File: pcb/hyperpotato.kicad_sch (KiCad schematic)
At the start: 38 parts, among them J1 Conn_01x02_Socket, J2 Conn_01x03_Pin, Q1 AO3401A, SW1 SW_Push_45deg, SW10 SW_Push_45deg, SW11 SW_Push_45deg, SW12 SW_Push_45deg, SW13 SW_Push_45deg, SW14 SW_SPDT, SW15 SW_Push, SW2 SW_Push_45deg, SW3 SW_Push_45deg, SW4 SW_Push_45deg, SW5 SW_Push_45deg, SW6 SW_Push_45deg, SW7 SW_Push_45deg, SW8 SW_Push_45deg, SW9 SW_Push_45deg, U1 Seeeduino Xiao nRF52840, U2 SK8707-01-SENSOR, U3 SK8707-01, U4 DRV2605LDGS

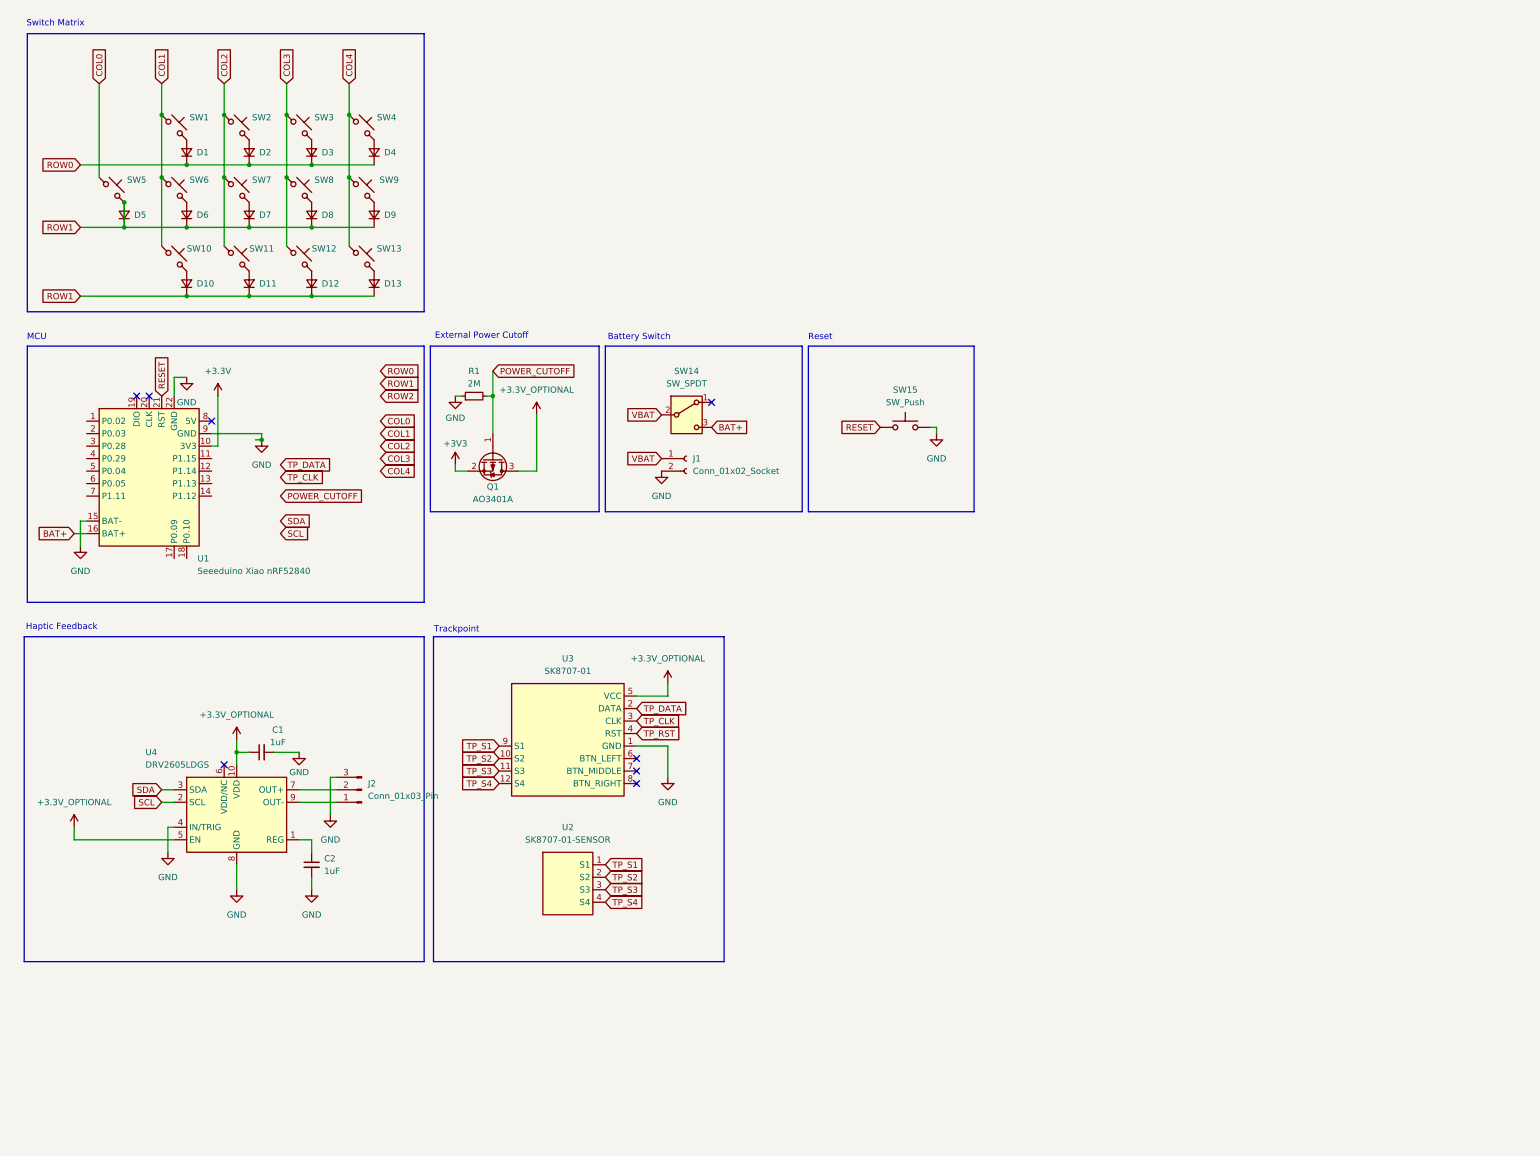
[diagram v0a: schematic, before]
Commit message: Start back with e73 module
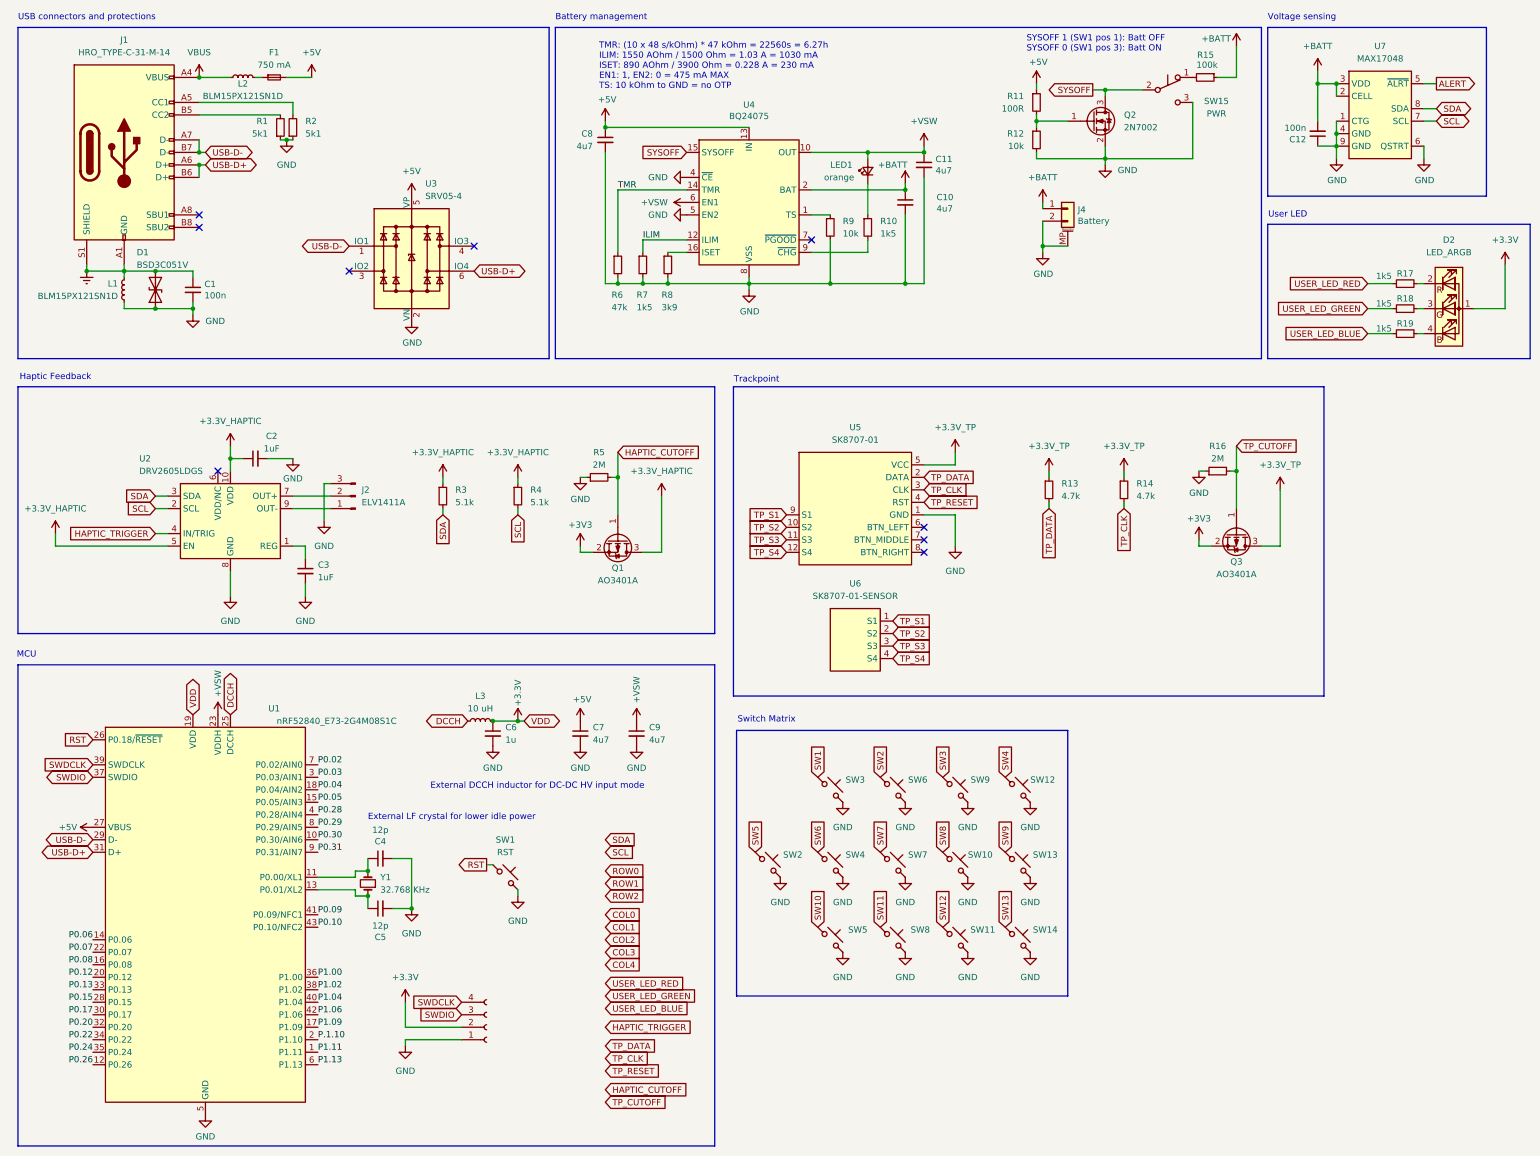
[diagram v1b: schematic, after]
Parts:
- removed D1, D10, D11, D12, D13, D2, D3, D4, D5, D6, D7, D8, D9: D_Small, ssbb_parts:D_1206_HandSolder_reversible, symbol Device:D_Small
- removed J1: Conn_01x02_Socket, ssbb_parts:JST_PH_S2B-PH-K_Horizontal_reversible, symbol Connector:Conn_01x02_Socket
- removed SW10, SW12: SW_Push_45deg, ssbb_parts:SW_choc_v1_reversible_1u, symbol Switch:SW_Push_45deg
- removed SW13: SW_Push_45deg, ssbb_parts:SW_choc_v1_reversible_1.5u, symbol Switch:SW_Push_45deg
- removed SW14: SW_SPDT, ssbb_parts:SW_SPDT_PCM12_reversible, symbol Switch:SW_SPDT
- removed SW15: SW_Push, ssbb_parts:Panasonic_EVQPUL_EVQPUC_reversible, symbol Switch:SW_Push
- removed U1: Seeeduino Xiao nRF52840, ssbb_parts:Xiao_nRF52840_AC_Reflow_reversible, symbol PCM_marbastlib-promicroish:Seeeduino_Xiao_nRF52840
- removed U2: SK8707-01-SENSOR, ssbb_parts:Sprintek_SK8707-01_Sensor, symbol ssbb_parts:Sprintek_SK8707-01_Sensor
- removed U3: SK8707-01, symbol ssbb_parts:Sprintek_SK8707–01
- added C1, C12: 100n, Capacitor_SMD:C_0402_1005Metric, symbol Device:C_Small
- added C10, C11, C7, C8, C9: 4u7, Capacitor_SMD:C_0402_1005Metric, symbol Device:C_Small
- added C4, C5: 12p, Capacitor_SMD:C_0402_1005Metric, symbol Device:C_Small
- added C6: 1u, Capacitor_SMD:C_0402_1005Metric, symbol Device:C_Small
- added D1: BSD3C051V, Diode_SMD:D_SOD-323, symbol Device:D_TVS
- added D2: LED_ARGB, symbol Device:LED_ARGB
- added F1: 750 mA, Fuse:Fuse_0603_1608Metric, symbol Device:Fuse_Small
- added J1: HRO_TYPE-C-31-M-14, Connector_USB:USB_C_Receptacle_HRO_TYPE-C-31-M-12, symbol Connector:USB_C_Receptacle_USB2.0
- added J3: Conn_01x04_Socket, symbol Connector:Conn_01x04_Socket
- added J4: Battery, PCM_marbastlib-various:Molex_Pico-EZmate_78171-0002_1x02-1MP_P1.20mm_Vertical, symbol Connector_Generic_MountingPin:Conn_01x02_MountingPin
- added L1, L2: BLM15PX121SN1D, Inductor_SMD:L_0402_1005Metric, symbol Device:L_Small
- added L3: 10 uH, Inductor_SMD:L_0603_1608Metric, symbol Device:L_Small
- added LED1: orange, LED_SMD:LED_0402_1005Metric, symbol Device:LED_Small
- added Q2: 2N7002, Package_TO_SOT_SMD:SOT-23, symbol Transistor_FET:2N7002
- added Q3: AO3401A, Package_TO_SOT_SMD:SOT-23, symbol Transistor_FET:AO3401A
- added R1, R2: 5k1, Resistor_SMD:R_0402_1005Metric, symbol Device:R_Small
- added R10, R7: 1k5, Resistor_SMD:R_0402_1005Metric, symbol Device:R_Small
- added R11: 100R, Resistor_SMD:R_0402_1005Metric, symbol Device:R_Small
- added R12, R9: 10k, Resistor_SMD:R_0402_1005Metric, symbol Device:R_Small
- added R13, R14: 4.7k, symbol Device:R_Small
- added R15: 100k, Resistor_SMD:R_0402_1005Metric, symbol Device:R_Small
- added R16: 2M, Resistor_SMD:R_0805_2012Metric, symbol Device:R_Small
- added R17, R18, R19: 1k5, symbol Device:R_Small
- added R3, R4: 5.1k, symbol Device:R_Small
- added R6: 47k, Resistor_SMD:R_0402_1005Metric, symbol Device:R_Small
- added R8: 3k9, Resistor_SMD:R_0402_1005Metric, symbol Device:R_Small
- added SW1: RST, PCM_marbastlib-various:SW_SPST_SKQG_WithStem, symbol Switch:SW_Push_45deg
- added SW14, SW2, SW8: SW_Push_45deg, symbol Switch:SW_Push_45deg
- added SW15: PWR, PCM_marbastlib-various:SW_MSK12C02-HB, symbol Switch:SW_Push_SPDT
- added U1: nRF52840_E73-2G4M08S1C, PCM_marbastlib-various:nRF52840_E73-2G4M08S1C, symbol PCM_marbastlib-various:nRF52840_E73-2G4M08S1C
- added U3: SRV05-4, Package_TO_SOT_SMD:SOT-23-6, symbol Power_Protection:SRV05-4
- added U4: BQ24075, Package_DFN_QFN:VQFN-16-1EP_3x3mm_P0.5mm_EP1.6x1.6mm, symbol Battery_Management:BQ24075RGT
- added U5: SK8707-01, symbol ssbb_parts:Sprintek_SK8707–01
- added U6: SK8707-01-SENSOR, ssbb_parts:Sprintek_SK8707-01_Sensor, symbol ssbb_parts:Sprintek_SK8707-01_Sensor
- added U7: MAX17048, Package_DFN_QFN:DFN-8-1EP_2x2mm_P0.5mm_EP0.7x1.3mm, symbol marbastlib-various:MAX17048
- added Y1: 32.768 KHz, Crystal:Crystal_SMD_2012-2Pin_2.0x1.2mm, symbol Device:Crystal_Small
- C2: renamed from C1; footprint ssbb_parts:C_1206_HandSolder_reversible -> (none)
- C3: renamed from C2; footprint ssbb_parts:C_1206_HandSolder_reversible -> (none)
- J2: value Conn_01x03_Pin -> ELV1411A
- SW10: renamed from SW8; footprint ssbb_parts:SW_choc_v1_reversible_1u -> (none)
- SW11, SW5, SW7: footprint ssbb_parts:SW_choc_v1_reversible_1u -> (none)
- SW12: renamed from SW4; footprint ssbb_parts:SW_choc_v1_reversible_1u -> (none)
- SW13: renamed from SW9; footprint ssbb_parts:SW_choc_v1_reversible_1u -> (none)
- SW3: renamed from SW1; footprint ssbb_parts:SW_choc_v1_reversible_1u -> (none)
- SW4: renamed from SW6; footprint ssbb_parts:SW_choc_v1_reversible_1u -> (none)
- SW6: renamed from SW2; footprint ssbb_parts:SW_choc_v1_reversible_1u -> (none)
- SW9: renamed from SW3; footprint ssbb_parts:SW_choc_v1_reversible_1u -> (none)
- renumbered R1 to R5, U4 to U2
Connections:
- net +3.3V: now also C6.1, D2.1 (A), J3.2 (Pin_2), L3.2, U1.19 (VDD)
- net +3V3: now also Q3.2 (S)
- net COL0: no longer SW5.1
- net COL1: no longer SW3.1, SW4.1
- net COL2: no longer SW11.1, SW6.1, SW7.1
- net COL3: no longer SW10.1, SW9.1
- net COL4: no longer SW12.1, SW13.1
- net GND: now also SW10.2, SW11.2, SW12.2, SW13.2, SW3.2, SW4.2, SW5.2, SW6.2, SW7.2, SW9.2, C1.2, C10.2, C11.2, C12.1, C4.2, C5.2, C6.2, C7.2, C8.2, C9.2, D1.1 (A1), J3.1 (Pin_1), J4.2 (Pin_2), J4.MP (MountPin), L1.2, Q2.2 (S), R1.1, R12.2, R16.1, R2.1, R6.2, R7.2, R8.2, R9.2, SW1.2, SW14.2, SW15.3 (C), SW2.2, SW8.2, U1.21 (GND), U1.24 (GND), U1.5 (GND), U3.2 (VN), U4.17 (VSS), U4.4 (~{CE}), U4.5 (EN2), U4.8 (VSS), U5.1 (GND), U7.1 (CTG), U7.4 (GND), U7.6 (QSTRT), U7.9 (GND); no longer U2.4 (IN/TRIG)
- net ROW1: no longer SW5.2
- net SCL: now also R4.2, U7.7 (SCL)
- net SDA: now also R3.2, U7.8 (SDA)
- net TP_CLK: now also R14.2, U5.3 (CLK)
- net TP_DATA: now also R13.2, U5.2 (DATA)
- net TP_S1: now also U5.9 (S1), U6.1 (S1)
- net TP_S2: now also U5.10 (S2), U6.2 (S2)
- net TP_S3: now also U5.11 (S3), U6.3 (S3)
- net TP_S4: now also U5.12 (S4), U6.4 (S4)
- net +3.3V_OPTIONAL renamed +3.3V_HAPTIC
- net +3.3V_HAPTIC: now also R3.1, R4.1
- net POWER_CUTOFF renamed HAPTIC_CUTOFF
- new net: J1.A5 (CC1), R2.2
- new net: C5.1, U1.13 (P0.01/XL2), Y1.1
- new net: C4.1, U1.11 (P0.00/XL1), Y1.2
- new net: F1.1, L2.2
- new net: J1.B5 (CC2), R1.2
- new net: Q2.1 (G), R11.2, R12.1
- new net: D2.2 (RK), R17.2
- new net: LED1.1 (K), R10.1
- new net: R10.2, U4.9 (~{CHG})
- new net: D2.3 (GK), R18.2
- new net: D2.4 (BK), R19.2
- new net: R15.2, SW15.1 (A)
- new net: R9.1, U4.1 (TS)
- new net: R8.1, U4.16 (ISET)
- new net +3.3V_TP: Q3.3 (D), R13.1, R14.1, U5.5 (VCC)
- new net +5V: C7.1, C8.1, F1.2, R11.1, U1.27 (VBUS), U3.5 (VP), U4.13 (IN)
- new net +BATT: C10.1, C12.2, J4.1 (Pin_1), R15.1, U4.2 (BAT), U4.3 (BAT), U7.2 (CELL), U7.3 (VDD)
- new net +VSW: C11.1, C9.1, LED1.2 (A), U1.23 (VDDH), U4.10 (OUT), U4.11 (OUT), U4.6 (EN1)
- new net ALERT: U7.5 (~{ALRT})
- new net DCCH: L3.1, U1.25 (DCCH)
- new net Earth: C1.1, D1.2 (A2), J1.A1 (GND), J1.A12 (GND), J1.B1 (GND), J1.B12 (GND), J1.S1 (SHIELD), L1.1
- new net HAPTIC_TRIGGER: U2.4 (IN/TRIG)
- new net ILIM: R7.1, U4.12 (ILIM)
- new net P.1.10: U1.2 (P1.10)
- new net P0.02: U1.7 (P0.02/AIN0)
- new net P0.03: U1.3 (P0.03/AIN1)
- new net P0.04: U1.18 (P0.04/AIN2)
- new net P0.05: U1.15 (P0.05/AIN3)
- new net P0.06: U1.14 (P0.06)
- new net P0.07: U1.22 (P0.07)
- new net P0.08: U1.16 (P0.08)
- new net P0.09: U1.41 (P0.09/NFC1)
- new net P0.10: U1.43 (P0.10/NFC2)
- new net P0.12: U1.20 (P0.12)
- new net P0.13: U1.33 (P0.13)
- new net P0.15: U1.28 (P0.15)
- new net P0.17: U1.30 (P0.17)
- new net P0.20: U1.32 (P0.20)
- new net P0.22: U1.34 (P0.22)
- new net P0.24: U1.35 (P0.24)
- new net P0.26: U1.12 (P0.26)
- new net P0.28: U1.4 (P0.28/AIN4)
- new net P0.29: U1.8 (P0.29/AIN5)
- new net P0.30: U1.10 (P0.30/AIN6)
- new net P0.31: U1.9 (P0.31/AIN7)
- new net P1.00: U1.36 (P1.00)
- new net P1.02: U1.38 (P1.02)
- new net P1.04: U1.40 (P1.04)
- new net P1.06: U1.42 (P1.06)
- new net P1.09: U1.17 (P1.09)
- new net P1.11: U1.1 (P1.11)
- new net P1.13: U1.6 (P1.13)
- new net RST: SW1.1, U1.26 (P0.18/~{RESET})
- new net SW1: SW3.1
- new net SW10: SW5.1
- new net SW11: SW8.1
- new net SW12: SW11.1
- new net SW13: SW14.1
- new net SW2: SW6.1
- new net SW3: SW9.1
- new net SW4: SW12.1
- new net SW5: SW2.1
- new net SW6: SW4.1
- new net SW7: SW7.1
- new net SW8: SW10.1
- new net SW9: SW13.1
- new net SWDCLK: J3.4 (Pin_4), U1.39 (SWDCLK)
- new net SWDIO: J3.3 (Pin_3), U1.37 (SWDIO)
- new net SYSOFF: Q2.3 (D), SW15.2 (B), U4.15 (SYSOFF)
- new net TMR: R6.1, U4.14 (TMR)
- new net TP_CUTOFF: Q3.1 (G), R16.2
- new net TP_RESET: U5.4 (RST)
- new net USB-D+: J1.A6 (D+), J1.B6 (D+), U1.31 (D+), U3.6 (IO4)
- new net USB-D-: J1.A7 (D-), J1.B7 (D-), U1.29 (D-), U3.1 (IO1)
- new net USER_LED_BLUE: R19.1
- new net USER_LED_GREEN: R18.1
- new net USER_LED_RED: R17.1
- new net VBUS: J1.A4 (VBUS), J1.A9 (VBUS), J1.B4 (VBUS), J1.B9 (VBUS), L2.1
- no-connect marks 8 -> 9
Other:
- note added: "Battery management"
- note added: "External DCCH inductor for DC-DC HV input mode"
- note added: "External LF crystal for lower idle power"
- note added: "SYSOFF 1 (SW1 pos 1): Batt OFF SYSOFF 0 (SW1 pos 3): Batt ON"
- note added: "TMR: (10 x 48 s/kOhm) * 47 kOhm = 22560s = 6.27h ILIM: 1550 AOhm / 1500 Ohm = 1.03 A = 1030 mA ISET: 890 AOhm / 3900 Ohm = 0.228 A = 230 mA EN1: 1, EN2: 0 = 475 mA MAX TS: 10 kOhm to GND = no OTP"
- note added: "USB connectors and protections"
- note added: "User LED"
- note added: "Voltage sensing"
- note removed: "Battery Switch"
- note removed: "External Power Cutoff"
- note removed: "Reset"
- moved on the sheet: C2, C3, Q1, R5, SW10, SW12, SW13, SW3, SW4, SW6, SW7, SW9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
